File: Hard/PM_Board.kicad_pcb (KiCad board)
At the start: 2 copper layers, 70 x 60 mm, 72 parts, among them J1 Micro_SD_Card_Det_Hirose_DM3AT, J101 LiPo_V+, J102 LiPo_V-, J2 KRC_Conn_SWD, J3 USB_B_Micro, J4 KRC_Conn_CAN, J5 KRC_Conn_CAN, J6 KRC_Conn_CAN, Q1 SSM6J501NU, Q2 2n7002, U1 CY8C58xxLTI-LPxxx, U2 INA226, U3 NCV7342, Y1 24MHz

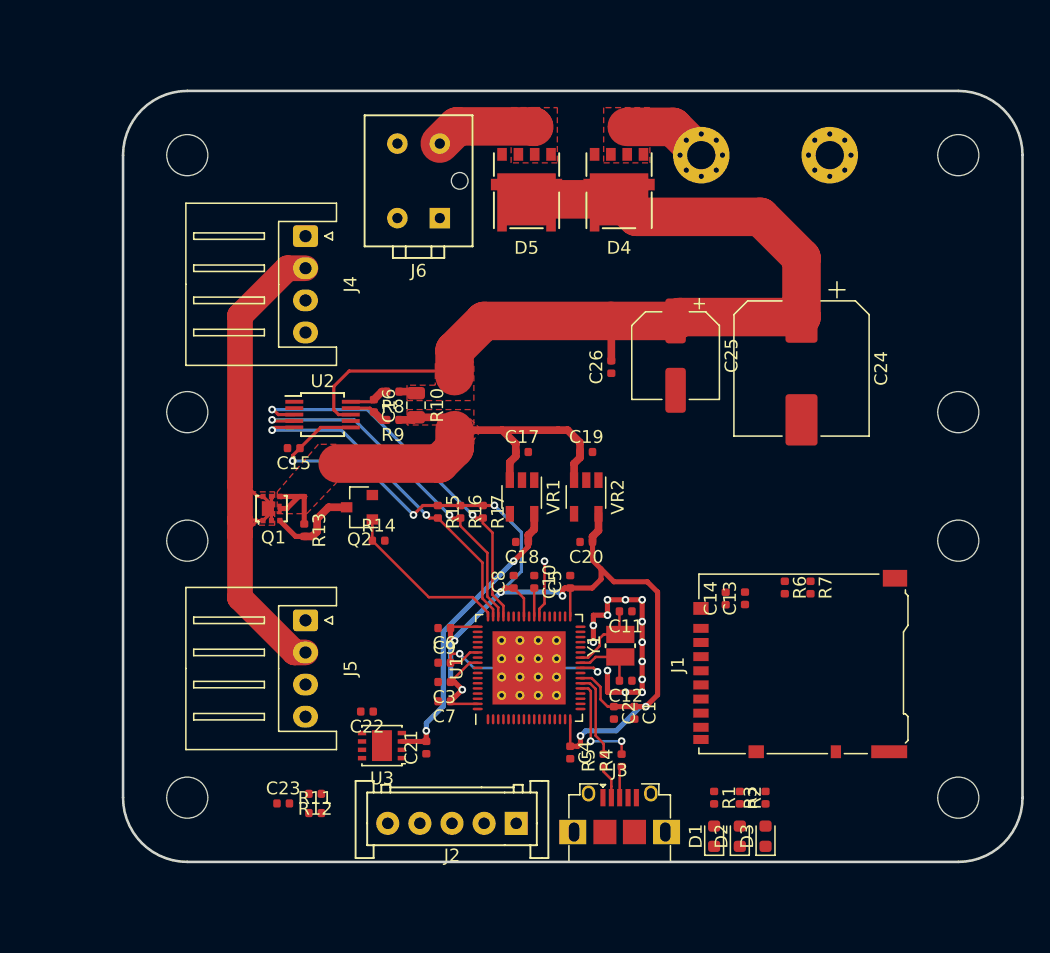
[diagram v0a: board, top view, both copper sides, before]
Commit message: [add] 基板完成
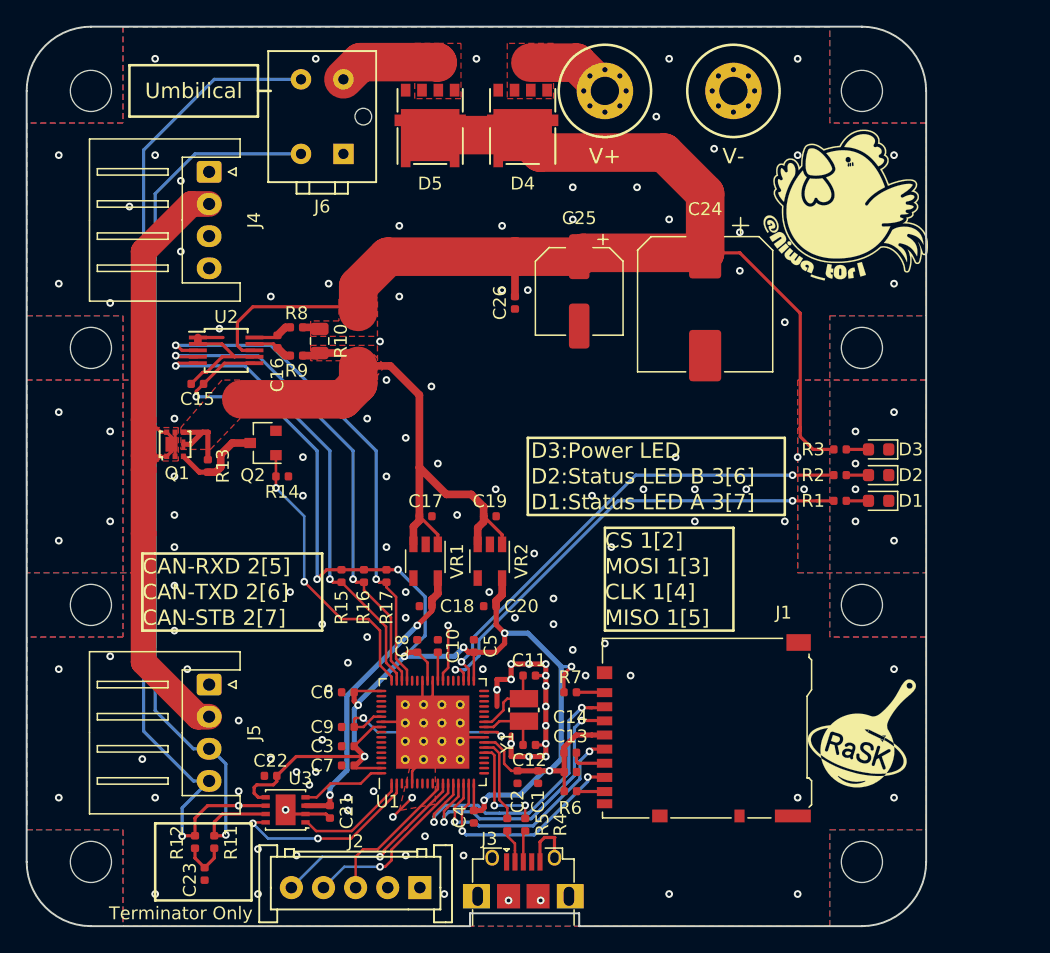
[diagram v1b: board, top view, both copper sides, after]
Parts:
- removed the REF** at (185.0, 100.0)
- removed the REF** at (125.0, 110.0)
- removed the REF** at (125.0, 100.0)
- removed the REF** at (185.0, 130.0)
- removed the REF** at (125.0, 130.0)
- removed the REF** at (185.0, 80.0)
- removed the REF** at (125.0, 80.0)
- added G***: LOGO, logo:Rask_sq, F.Cu at (177.5, 125.0)
- added G***: LOGO, logo:niwatori, F.Cu at (176.2, 83.8)
- added G***: LOGO, logo:arrows, B.Cu at (156.5, 81.0)
- added REF**: MountingHole_3.2mm_M3, MountingHole:MountingHole_3.2mm_M3, F.Cu at (177.5, 95.0)
- added REF**: MountingHole_3.2mm_M3, MountingHole:MountingHole_3.2mm_M3, F.Cu at (117.5, 115.0)
- added REF**: MountingHole_3.2mm_M3, MountingHole:MountingHole_3.2mm_M3, F.Cu at (117.5, 95.0)
- added REF**: MountingHole_3.2mm_M3, MountingHole:MountingHole_3.2mm_M3, F.Cu at (177.5, 75.0)
- added REF**: MountingHole_3.2mm_M3, MountingHole:MountingHole_3.2mm_M3, F.Cu at (177.5, 135.0)
- added REF**: MountingHole_3.2mm_M3, MountingHole:MountingHole_3.2mm_M3, F.Cu at (117.5, 135.0)
- added REF**: MountingHole_3.2mm_M3, MountingHole:MountingHole_3.2mm_M3, F.Cu at (117.5, 75.0)
- moved D3 31.4 mm to (178.8, 102.9), turned to 180 degrees
- moved D2 30.1 mm to (178.8, 104.9), turned to 180 degrees
- moved D1 29.1 mm to (178.8, 106.9), turned to 180 degrees
- moved R3 27.7 mm to (175.8, 102.9), turned to 180 degrees
- moved R2 26.3 mm to (175.8, 104.9), turned to 0 degrees
- moved R1 25.1 mm to (175.8, 106.9), turned to 0 degrees
- moved R6 23.0 mm to (154.8, 129.5), turned to 0 degrees
- moved R7 20.4 mm to (154.8, 121.8), turned to 0 degrees
- moved C13 19.2 mm to (154.8, 128.0), turned to 0 degrees
- moved C14 17.0 mm to (154.8, 126.5), turned to 0 degrees
- moved R12 10.1 mm to (125.6, 133.4), turned to 270 degrees
- moved Q1 9.01 mm to (124.0, 102.5)
- moved C22 9.01 mm to (131.5, 128.3), turned to 0 degrees
- moved C4 9.01 mm to (147.3, 131.5)
- moved C1 9.01 mm to (152.3, 128.4)
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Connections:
- U1 pad 13: Net-(U1-Pad13) -> /SD_CS
- U1 pad 14: Net-(U1-Pad14) -> /SD_MOSI
- U1 pad 15: Net-(U1-Pad15) -> /SD_CLK
- U1 pad 16: Net-(U1-Pad16) -> /SD_MISO
- U1 pad 2: /CAN_RXD -> /CAN_STB
- U1 pad 29: Net-(R2-Pad1) -> Net-(U1-Pad29)
- U1 pad 30: Net-(R1-Pad1) -> Net-(U1-Pad30)
- U1 pad 36: /SD_MISO -> Net-(R2-Pad1)
- U1 pad 37: /SD_CLK -> Net-(R1-Pad1)
- U1 pad 38: /SD_MOSI -> Net-(U1-Pad38)
- U1 pad 39: /SD_CS -> Net-(U1-Pad39)
- U1 pad 68: /CAN_STB -> /CAN_RXD
- U3 pad 9: (no net) -> GND
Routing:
- net /CAN_L: track 0.00 -> 79.9 mm, vias 0 -> 2
- net /CAN_H: track 0.00 -> 77.2 mm, vias 0 -> 1
- net GND: track 18.7 -> 56.1 mm, vias 13 -> 134
- net Net-(R2-Pad1): track 0.00 -> 37.3 mm, vias 0 -> 2
- net Net-(R1-Pad1): track 0.00 -> 37.0 mm, vias 0 -> 2
- net +3V3: track 103.0 -> 134.8 mm, vias 9 -> 11
- net /SD_CS: track 0.00 -> 24.0 mm, vias 0 -> 2
- net VCC: track 94.2 -> 116.9 mm
- net /SD_MOSI: track 0.00 -> 22.1 mm, vias 0 -> 2
- net /SD_CLK: track 0.00 -> 18.4 mm, vias 0 -> 2
- net /SD_MISO: track 0.00 -> 17.2 mm, vias 0 -> 2
- net Net-(J2-Pad5): track 0.00 -> 15.9 mm, vias 0 -> 1
- net /CAN_STB: track 0.00 -> 14.9 mm, vias 0 -> 2
- net Net-(C17-Pad1): track 39.7 -> 54.4 mm
- net Net-(J2-Pad4): track 0.00 -> 14.0 mm, vias 0 -> 1
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- added copper zone on B.Cu, net GND
- added copper zone on F.Cu, net GND
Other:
- board size 70 x 60 mm -> 70 x 70 mm
- board text added: "CAN-H"
- board text added: "CAN-L"
- board text added: "CAN-RXD 2[5]"
- board text added: "CAN-STB 2[7]"
- board text added: "CAN-TXD 2[6]"
- board text added: "CLK"
- board text added: "CLK 1[4]"
- board text added: "CS 1[2]"
- board text added: "D1:Status LED A 3[7]"
- board text added: "D2:Status LED B 3[6]"
- board text added: "D3:Power LED"
- board text added: "DIO"
- board text added: "Date"
- board text added: "GND"
- board text added: "GS-8 PM Board Rev.1 Designed by T.Niwa 2019.9"
- board text added: "MISO 1[5]"
- board text added: "MOSI 1[3]"
- board text added: "Manufacturer"
- board text added: "NC"
- board text added: "Note"
- board text added: "RES"
- board text added: "Terminator Only"
- board text added: "Umbilical"
- board text added: "V+"
- board text added: "V-"
- board text added: "VCC"
